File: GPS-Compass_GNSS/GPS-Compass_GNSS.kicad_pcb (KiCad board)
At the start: 2 copper layers, 40.5 x 29.6 mm, 38 parts, among them J3 01x10, J4 636101112001, Q1 MMBT3904, SW1 GNSS_RST, U1 BGA725L6E6327FTSA1, U2 TESEO-LIV3R

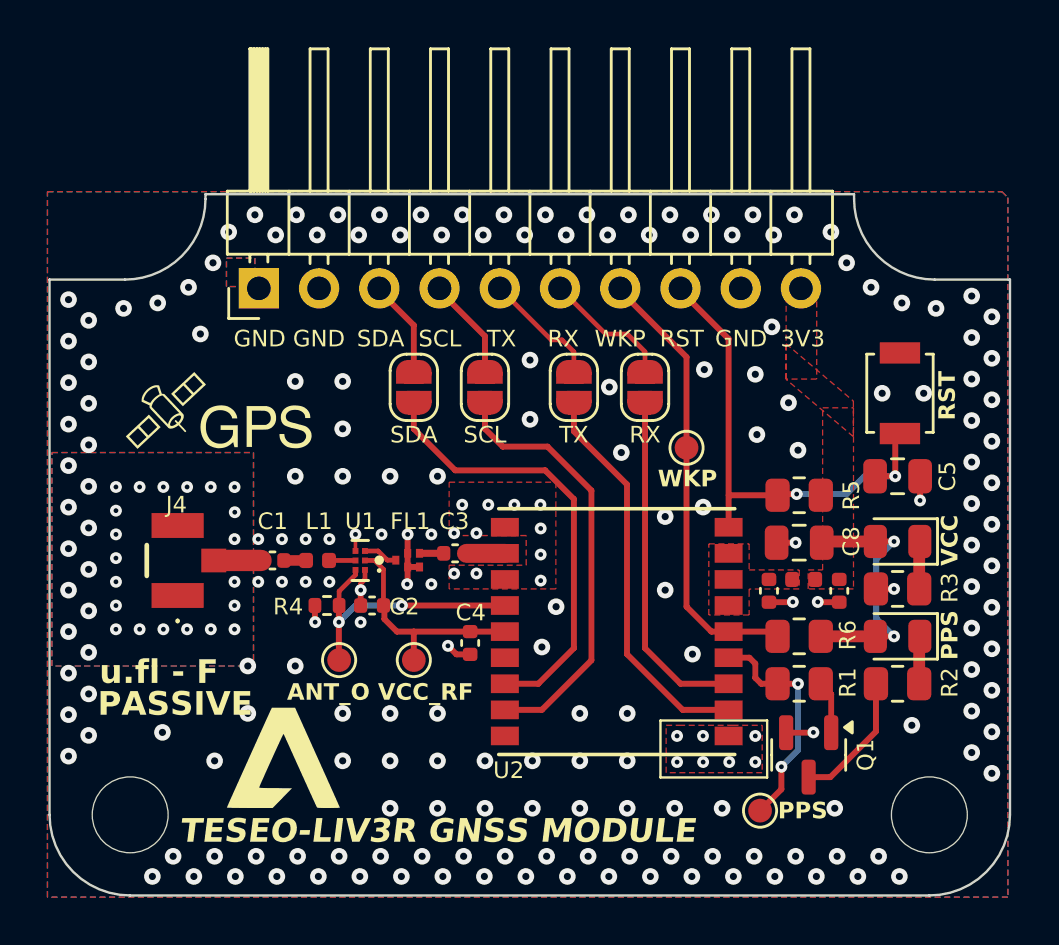
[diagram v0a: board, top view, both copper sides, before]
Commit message: new renders
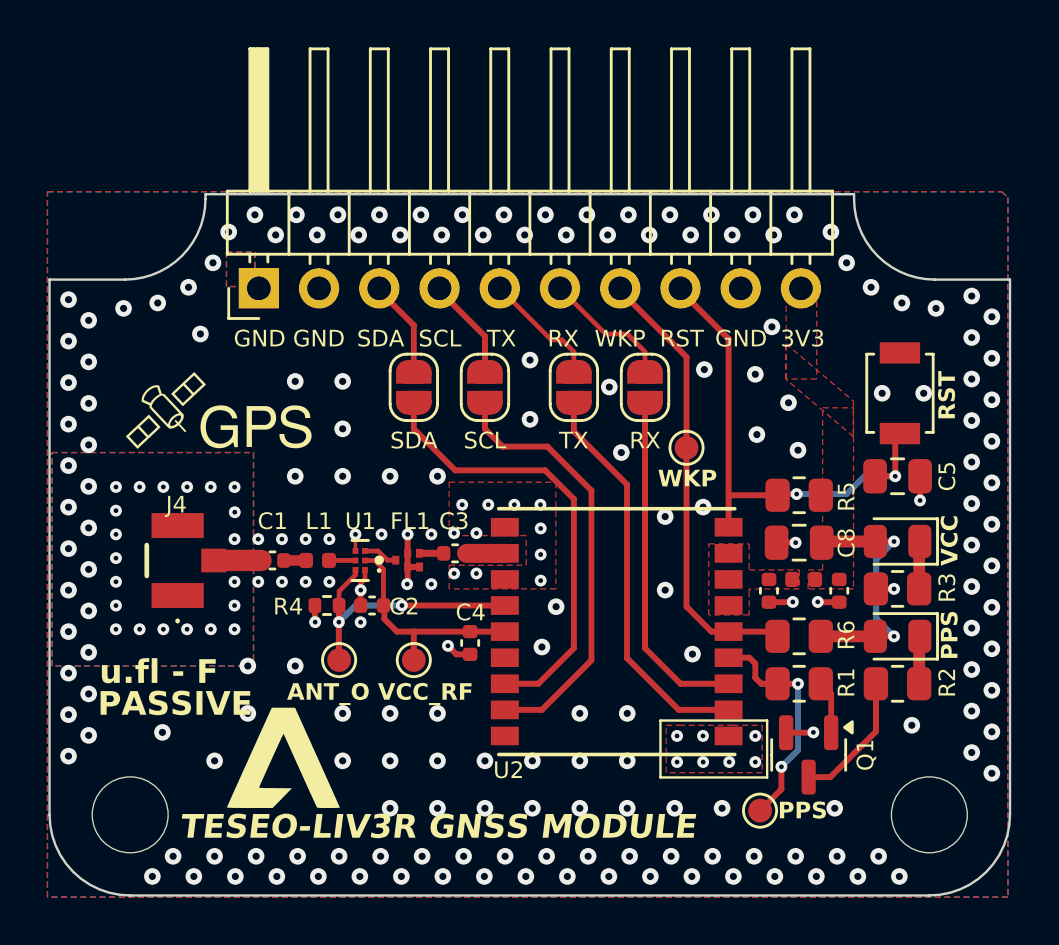
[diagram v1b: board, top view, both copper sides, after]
